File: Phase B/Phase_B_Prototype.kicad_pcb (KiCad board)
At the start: 2 copper layers, 99.1 x 71.1 mm, 48 parts, among them J1 USB_B_Mini, J3 AVR-ISP-6, J4 ESP_Conn, U1 CA56-12EWA, U2 74HC595, U3 ATmega32U4-A, U4 USBLC6-2SC6, U5 LP2985-3.3, Y1 16MHz

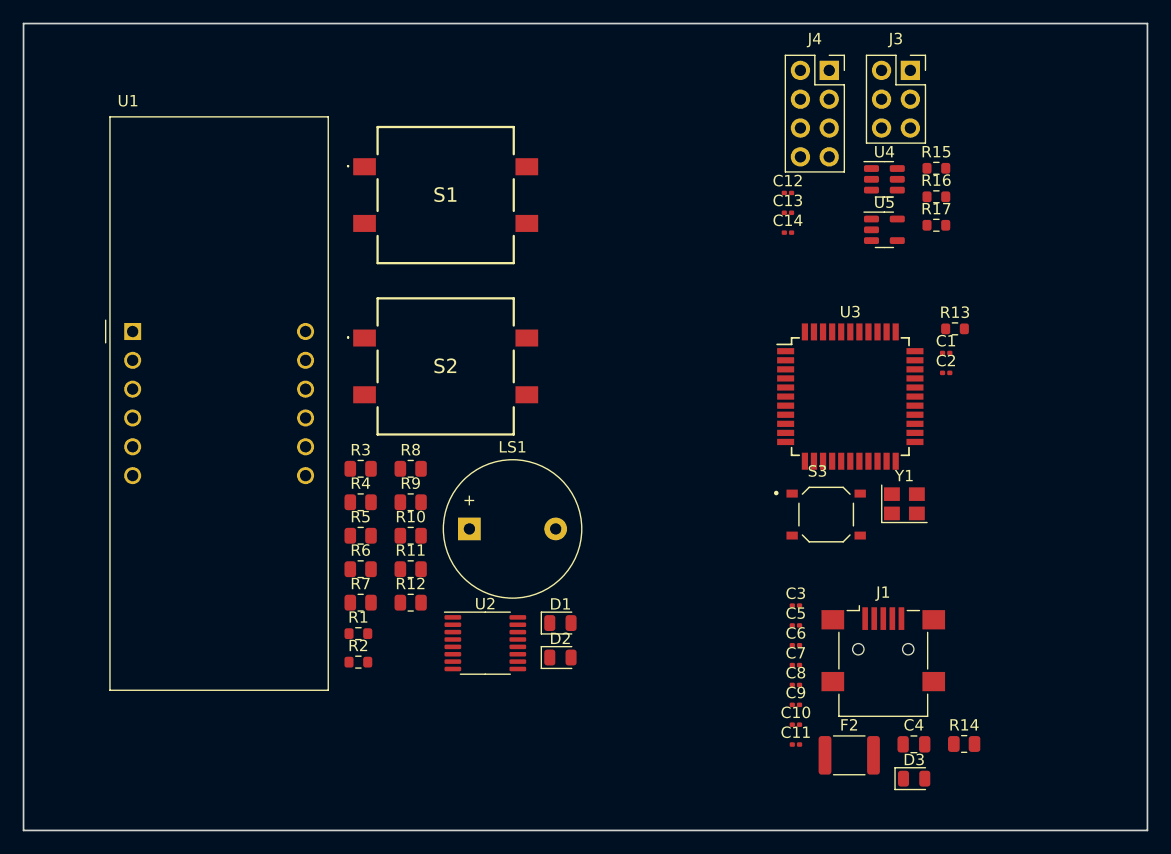
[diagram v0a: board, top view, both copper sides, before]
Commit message: Updated
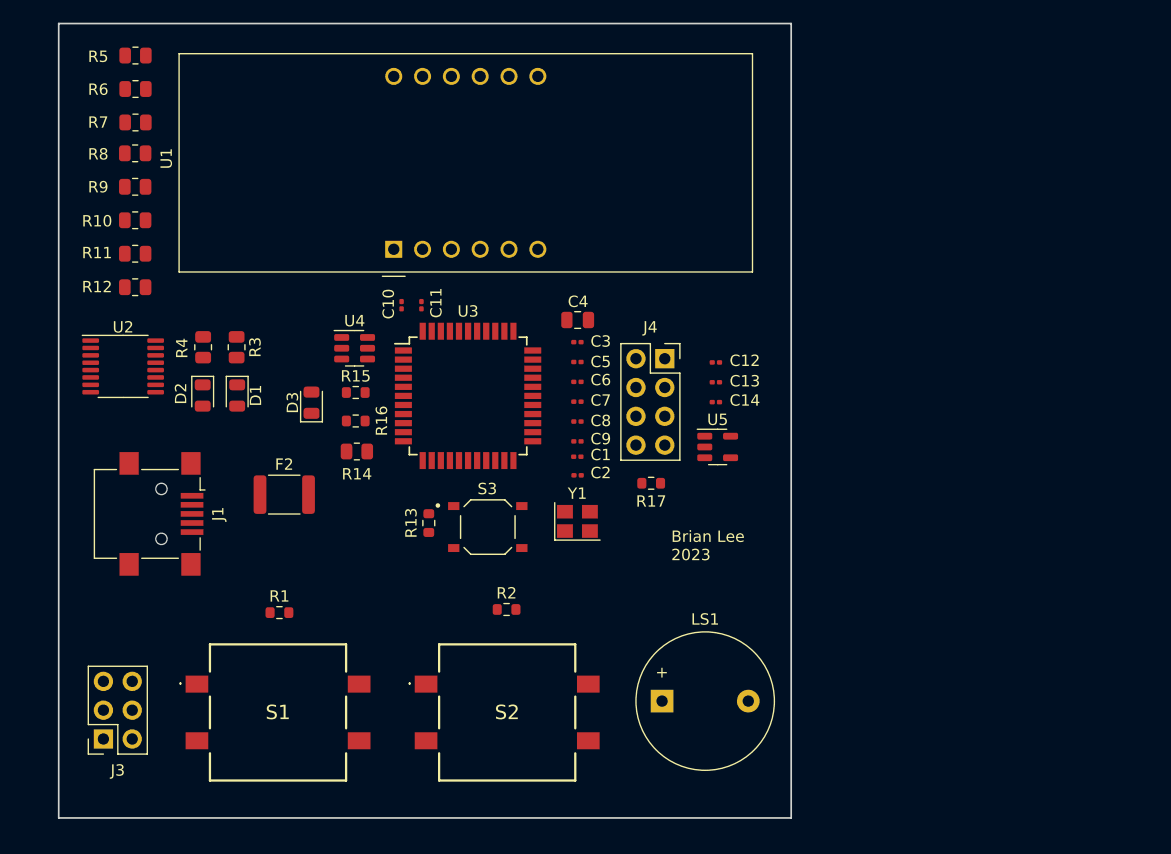
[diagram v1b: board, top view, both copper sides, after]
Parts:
- moved J3 92.4 mm to (116.3, 118.9), turned to 180 degrees
- moved J1 64.7 mm to (121.4, 99.1), turned to -90 degrees
- moved D3 62.6 mm to (134.6, 89.3), turned to 90 degrees
- moved R14 59.4 mm to (138.6, 93.6)
- moved R15 54.9 mm to (138.5, 88.4)
- moved R16 54.9 mm to (138.5, 90.9)
- moved F2 54.8 mm to (132.2, 97.4)
- moved C11 50.9 mm to (144.3, 80.7), turned to 90 degrees
- moved C10 50.7 mm to (142.5, 80.7), turned to 90 degrees
- moved R13 49.4 mm to (144.9, 99.9), turned to 90 degrees
- moved U4 49.0 mm to (138.4, 84.5)
- moved S1 47.9 mm to (131.7, 116.6)
- moved C4 47.7 mm to (158.1, 82.0)
- moved R5 46.7 mm to (119.1, 58.7)
- moved R7 46.7 mm to (119.1, 64.6)
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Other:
- board size 99.1 x 71.1 mm -> 64.6 x 70 mm
- board text added: "Brian Lee 2023"
- board text added: "Embedded Systems Kitchen Timer"
